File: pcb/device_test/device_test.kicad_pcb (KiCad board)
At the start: 4 copper layers, 80 x 80 mm, 24 parts, among them J101 Screw_Terminal_01x02, J201 USB_C_Receptacle_USB2.0_16P, J202 Conn_01x04, J203 Conn_02x10_Row_Letter_First, J301 USB_C_Receptacle_USB2.0_16P, J302 Conn_02x10_Row_Letter_First

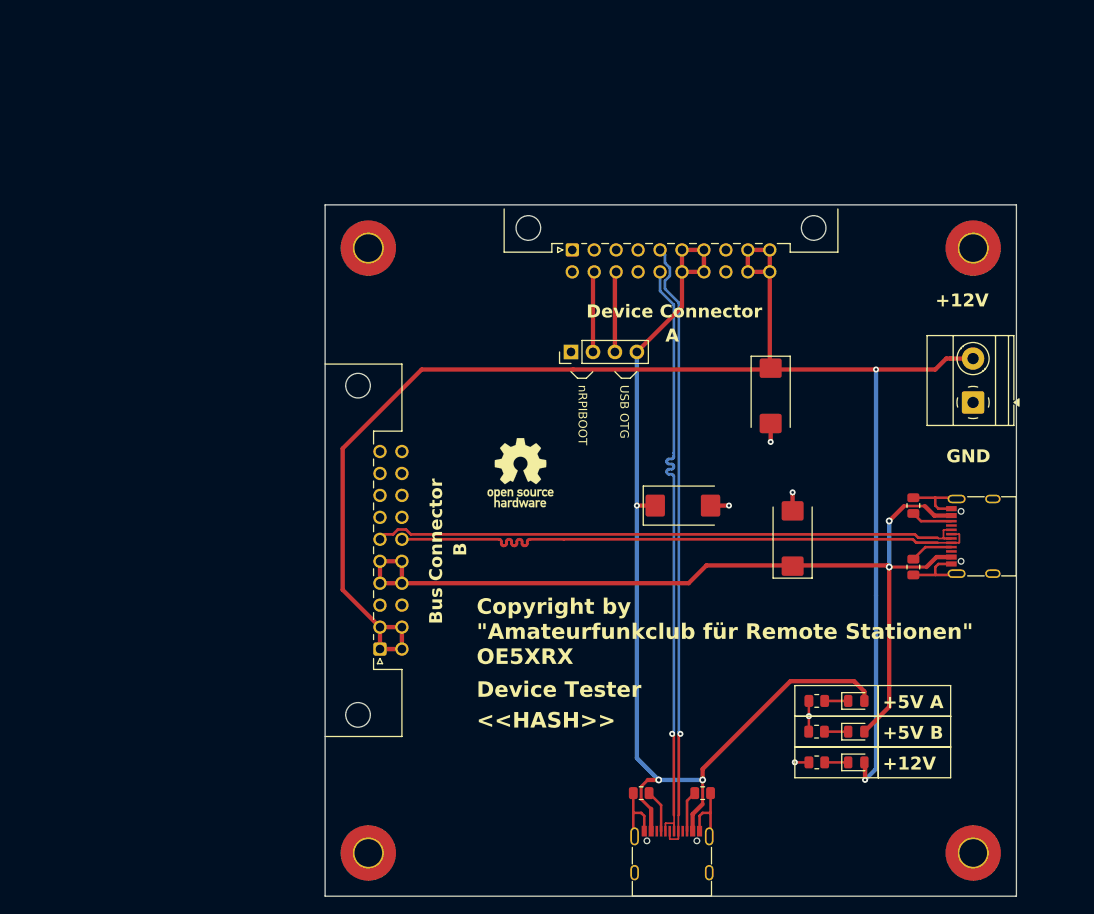
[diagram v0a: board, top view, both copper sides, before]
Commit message: fixes
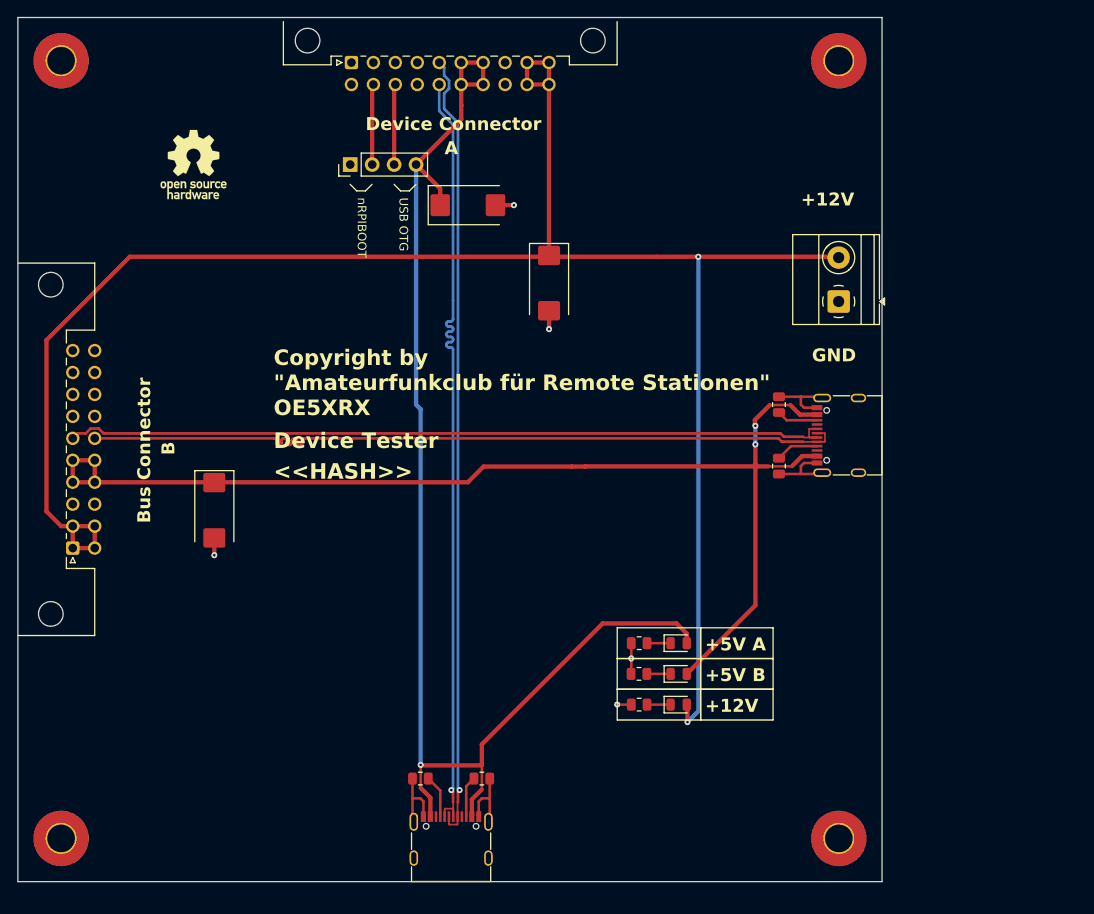
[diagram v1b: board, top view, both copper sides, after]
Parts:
- moved C301 67.0 mm to (102.9, 98.6), turned to -90 degrees
- moved #SYM101 52.0 mm to (100.5, 58.6)
- moved C201 42.8 mm to (132.3, 63.3)
- moved REF** 41.6 mm to (85.2, 46.6)
- moved J302 37.4 mm to (86.6, 103.0)
- moved REF** 35.6 mm to (85.2, 136.6)
- moved J203 33.5 mm to (118.8, 46.8)
- moved J202 33.5 mm to (118.7, 58.6)
- moved C101 28.8 mm to (141.7, 72.3)
- moved REF** 26.7 mm to (175.2, 46.6)
- moved R201 25.6 mm to (126.8, 129.6)
- moved R202 25.6 mm to (133.9, 129.6)
- moved J201 25.6 mm to (130.3, 137.8)
- moved R303 21.6 mm to (152.1, 117.5)
- moved D201 21.6 mm to (156.7, 114.0)
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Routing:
- net +12V: track 181.4 -> 216.0 mm
- net +5V_A: track 119.6 -> 150.7 mm, vias 3 -> 1
- net +5V_B: track 109.1 -> 136.3 mm
- net /Device Tester Connector/USB-: track 70.7 -> 91.6 mm
- net /Device Tester Connector/USB+: track 71.6 -> 91.7 mm
- net /Bus Tester Connector/USB-: track 69.7 -> 89.7 mm
- net /Bus Tester Connector/USB+: track 69.8 -> 89.8 mm
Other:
- board size 80 x 80 mm -> 100 x 100 mm
